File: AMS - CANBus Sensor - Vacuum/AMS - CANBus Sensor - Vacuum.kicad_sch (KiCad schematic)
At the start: 16 parts, among them J1 Power_And_CAN, J2 Power_And_CAN, J6 Screw_Terminal_01x02, Q1 IRF9Z34NPBF, U1 3568, U5 3568

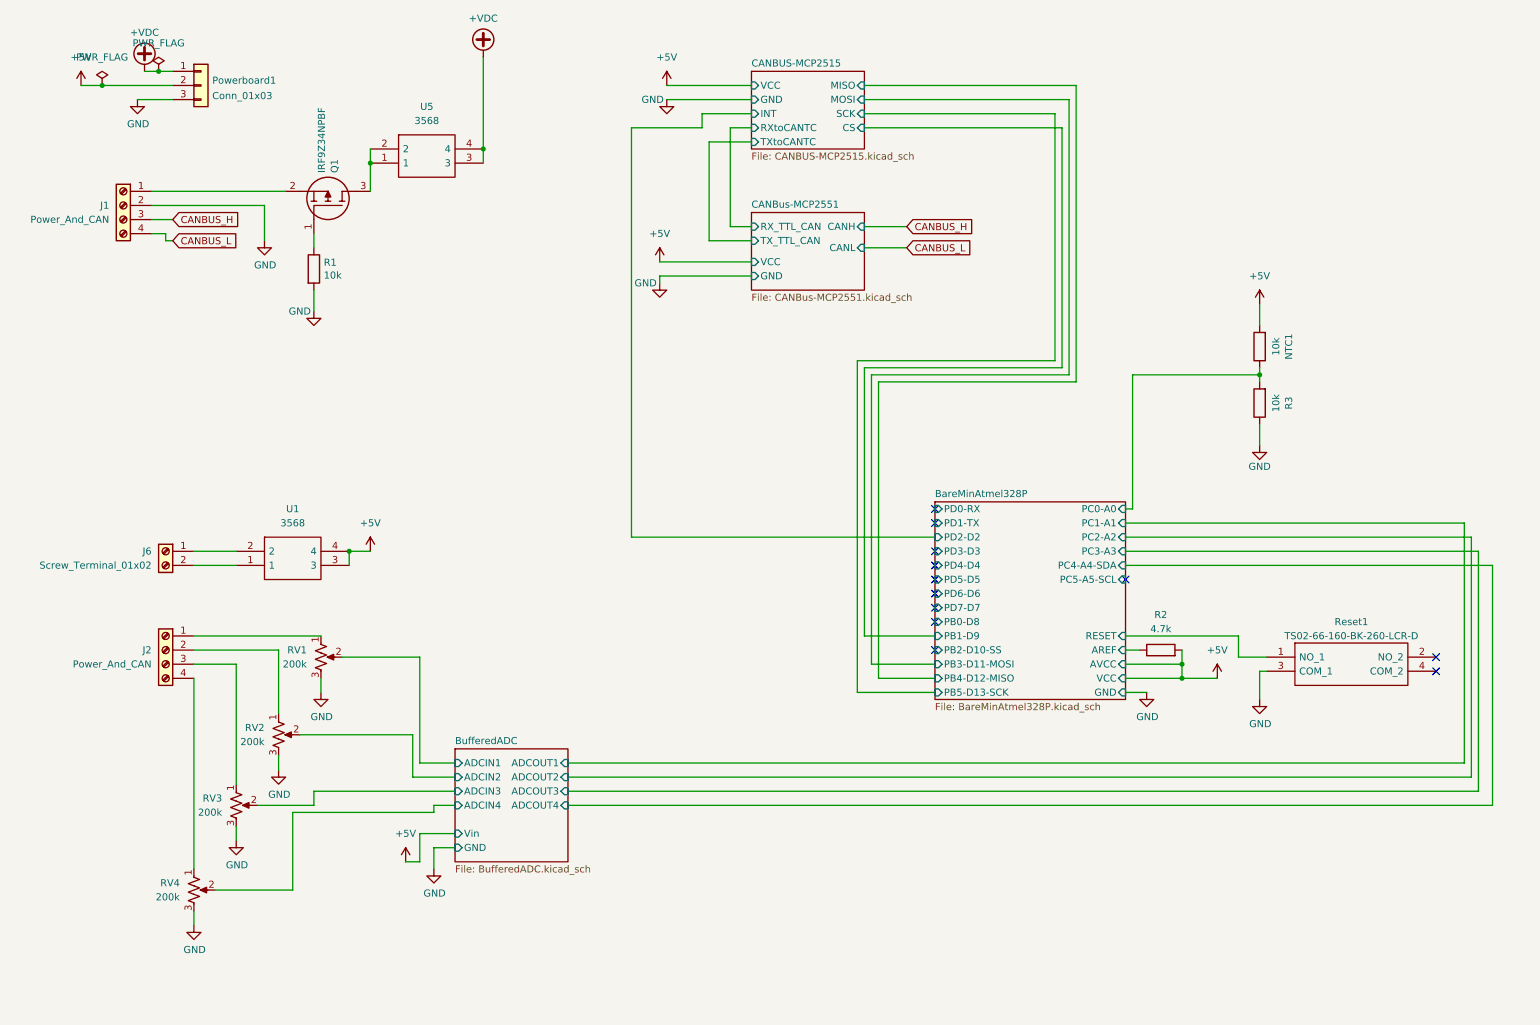
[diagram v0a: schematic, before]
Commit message: wip for the vacuum
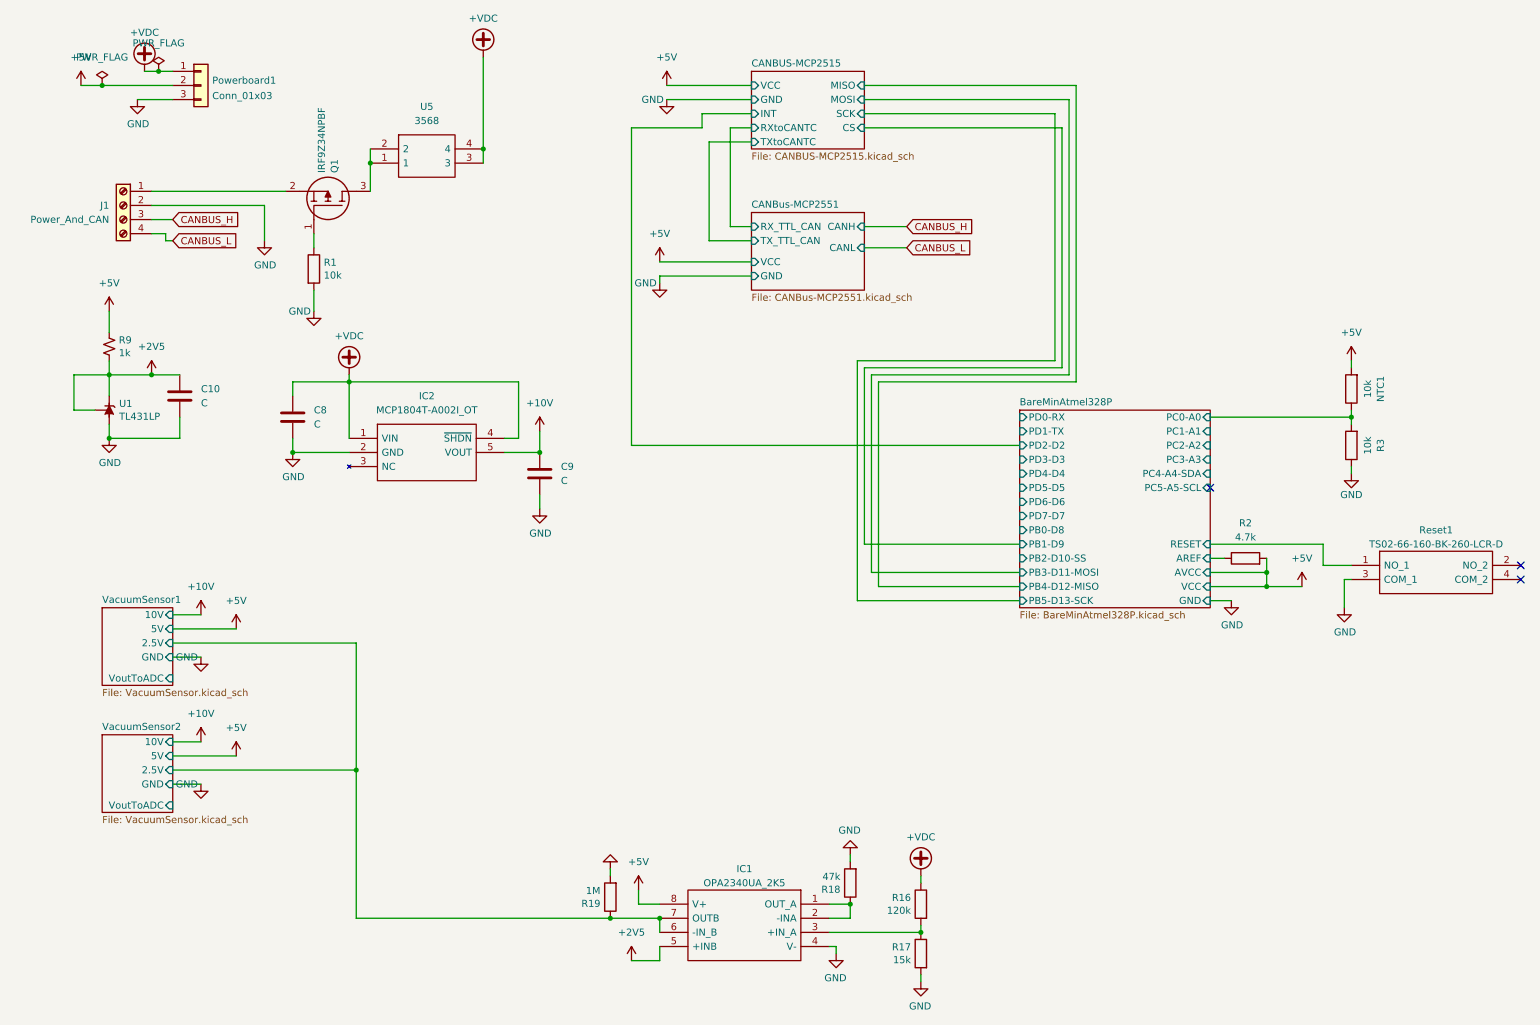
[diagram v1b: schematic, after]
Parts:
- removed J2: Power_And_CAN, TerminalBlock_Phoenix:TerminalBlock_Phoenix_MPT-0,5-4-2.54_1x04_P2.54mm_Horizontal, symbol Connector:Screw_Terminal_01x04
- removed J6: Screw_Terminal_01x02, TerminalBlock_Phoenix:TerminalBlock_Phoenix_MPT-0,5-2-2.54_1x02_P2.54mm_Horizontal, symbol Connector:Screw_Terminal_01x02
- removed RV1, RV2, RV3, RV4: 200k, Potentiometer_THT:Potentiometer_Bourns_3296W_Vertical, symbol Device:R_Potentiometer_US
- removed U1: 3568, 3568, symbol SamacSys_Parts:3568
- added C10, C8, C9: C, symbol Device:C
- added IC1: OPA2340UA_2K5, SamacSys_Parts:SOIC127P600X175-8N, symbol SamacSys_Parts:OPA2340UA_2K5
- added IC2: MCP1804T-A002I_OT, SOT95P270X145-5N, symbol SamacSys_Parts:MCP1804T-A002I_OT
- added R16: 120k, Resistor_SMD:R_1206_3216Metric_Pad1.30x1.75mm_HandSolder, symbol Device:R
- added R17: 15k, Resistor_SMD:R_1206_3216Metric_Pad1.30x1.75mm_HandSolder, symbol Device:R
- added R18: 47k, Resistor_SMD:R_1206_3216Metric_Pad1.30x1.75mm_HandSolder, symbol Device:R
- added R19: 1M, Resistor_SMD:R_1206_3216Metric_Pad1.30x1.75mm_HandSolder, symbol Device:R
- added R9: 1k, Resistor_SMD:R_0603_1608Metric, symbol Device:R_Small_US
- added U1: TL431LP, Package_TO_SOT_THT:TO-92_Inline, symbol Reference_Voltage:TL431LP
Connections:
- net +5V: now also IC1.8 (V+), R9.1
- net +VDC: now also C8.1, IC2.1 (VIN), IC2.4 (~{SHDN}), R16.1
- net GND: now also C10.2, C8.2, C9.2, IC1.4 (V-), IC2.2 (GND), R17.2, R18.2, R19.2, U1.2 (A)
- new net: IC1.1 (OUT_A), IC1.2 (-INA), R18.1
- new net: IC1.3 (+IN_A), R16.2, R17.1
- new net +10V: C9.1, IC2.5 (VOUT)
- new net +2V5: C10.1, IC1.5 (+INB), R9.2, U1.1 (REF), U1.3 (K)
- new net VacuumSensor1/2.5V: IC1.6 (-IN_B), IC1.7 (OUTB), R19.1
- no-connect marks 12 -> 3
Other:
- removed sheet BufferedADC
- added sheet VacuumSensor1 (VacuumSensor.kicad_sch)
- added sheet VacuumSensor2 (VacuumSensor.kicad_sch)
- moved on the sheet: NTC1, R2, R3, Reset1
